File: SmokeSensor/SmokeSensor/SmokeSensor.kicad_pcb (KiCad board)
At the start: 2 copper layers, 88.9 x 59.7 mm, 53 parts, among them J1 USB_C_Receptacle_USB2.0_16P, J2 Conn_01x05_Pin, J3 Conn_01x11, J4 Conn_01x04, Q1 SS8050, Q2 SS8050, SW1 RESET, SW2 BOOT, U1 MT3608, U2 TP4056-42-ESOP8, U3 MCP1700x-330xxMB, U4 CH340C, U5 SHT31-DIS, U6 ESP32-WROOM-32E

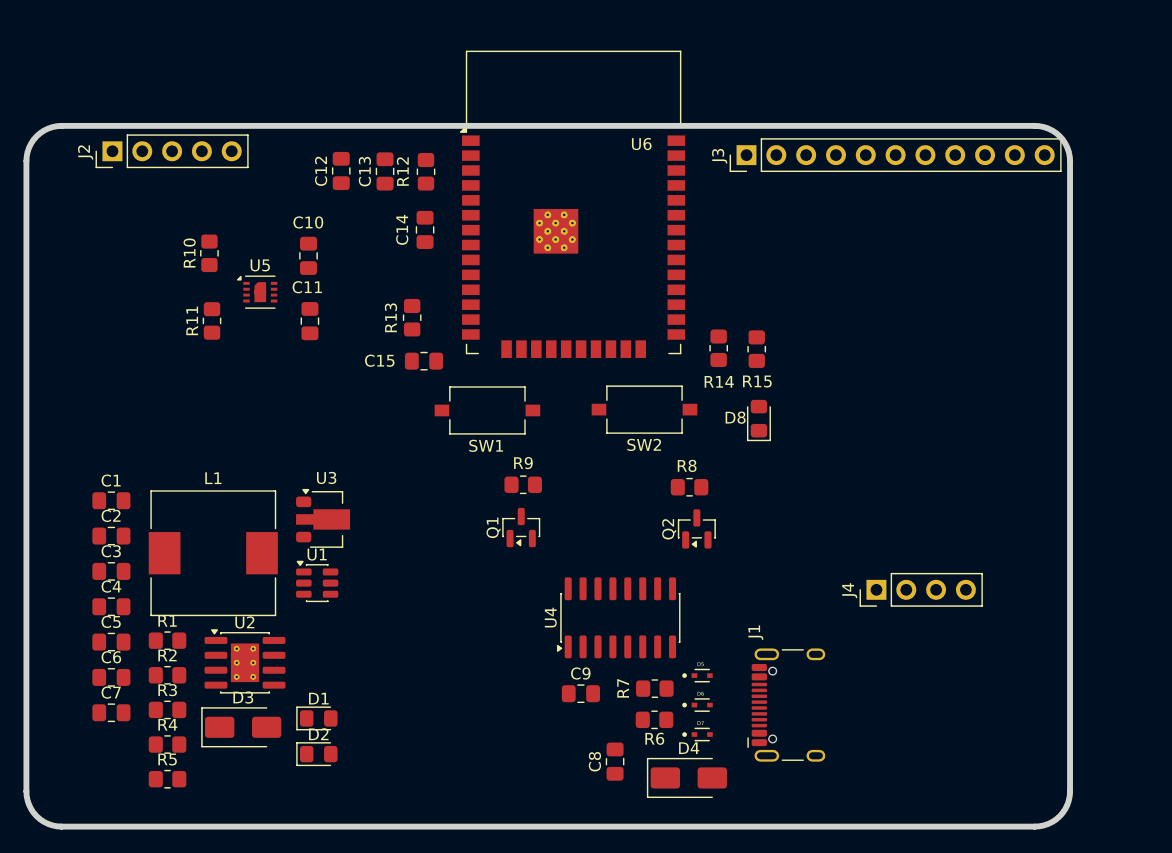
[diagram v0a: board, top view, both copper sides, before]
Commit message: layout 2-layers done!
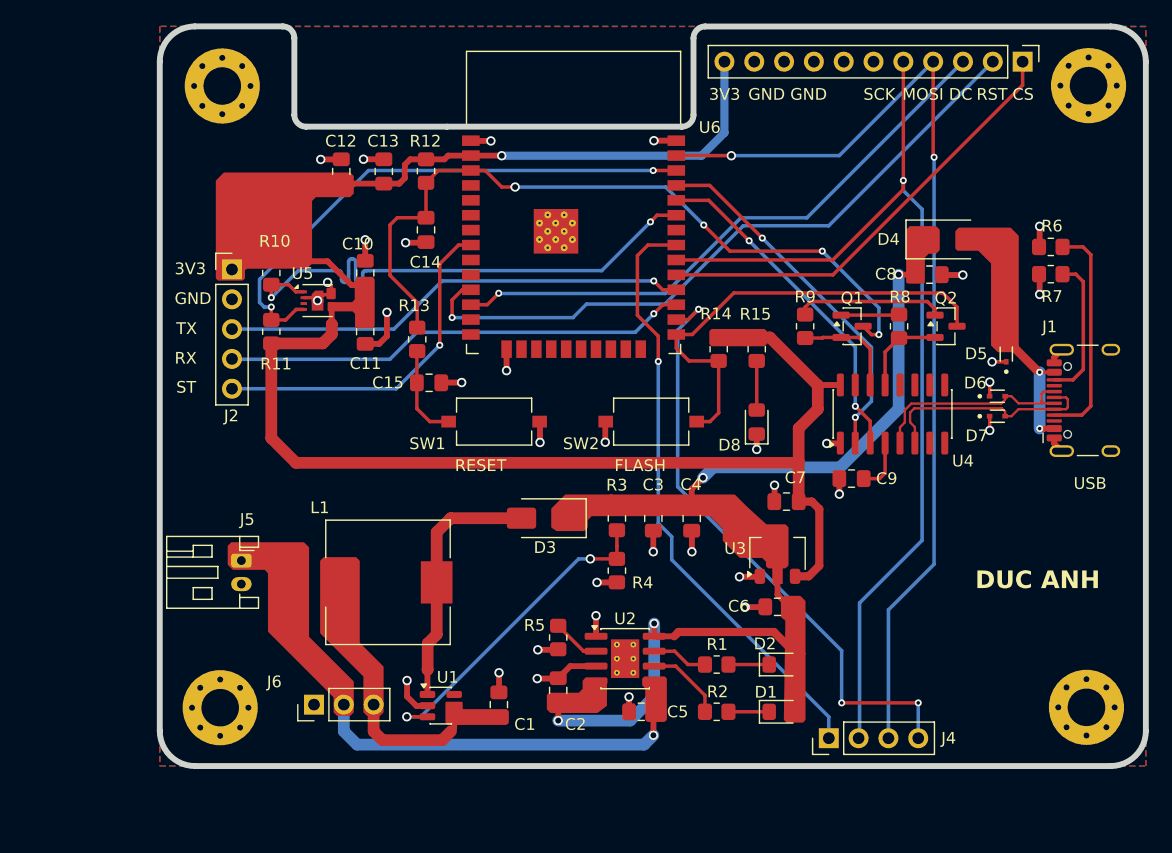
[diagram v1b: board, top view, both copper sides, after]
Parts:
- added J5: Pin lithium, Connector_JST:JST_PH_S2B-PH-K_1x02_P2.00mm_Horizontal, F.Cu at (122.5, 114.5)
- added J6: Switch, Connector_PinHeader_2.54mm:PinHeader_1x03_P2.54mm_Vertical, F.Cu at (128.6, 126.8)
- added REF**: MountingHole_3.2mm_M3_Pad_Via, MountingHole:MountingHole_3.2mm_M3_Pad_Via, F.Cu at (194.6, 74.0)
- added REF**: MountingHole_3.2mm_M3_Pad_Via, MountingHole:MountingHole_3.2mm_M3_Pad_Via, F.Cu at (194.4, 127.0)
- added REF**: MountingHole_3.2mm_M3_Pad_Via, MountingHole:MountingHole_3.2mm_M3_Pad_Via, F.Cu at (120.6, 127.0)
- added REF**: MountingHole_3.2mm_M3_Pad_Via, MountingHole:MountingHole_3.2mm_M3_Pad_Via, F.Cu at (120.8, 74.1)
- L1: value 22uH -> 22uH/2A
- R3: value 1k2 -> 100k
- R4: value 1k2 -> 2k2
- moved C7 60.3 mm to (168.9, 109.5), turned to 180 degrees
- moved C6 57.1 mm to (168.1, 118.4), turned to 180 degrees
- moved R6 52.6 mm to (191.4, 87.8)
- moved D4 50.9 mm to (182.6, 87.1)
- moved C4 50.0 mm to (160.8, 110.9), turned to -90 degrees
- moved C8 49.4 mm to (181.1, 90.1), turned to 0 degrees
- moved R7 48.8 mm to (191.4, 90.1)
- moved R2 46.9 mm to (162.9, 127.4), turned to 180 degrees
- moved R1 46.8 mm to (162.9, 123.4), turned to 180 degrees
- moved C3 46.4 mm to (157.5, 110.9), turned to -90 degrees
- moved C5 45.5 mm to (156.5, 127.4), turned to 180 degrees
- moved R3 41.6 mm to (154.4, 110.9), turned to 90 degrees
- moved R4 41.0 mm to (154.4, 115.4), turned to 90 degrees
- moved C2 40.3 mm to (149.4, 125.6), turned to 90 degrees
- moved D2 40.1 mm to (168.4, 123.4)
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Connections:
- net Net-(U1-EN) renamed /POWER/VBATT/PWR
- net Net-(U2-BAT) renamed /POWER/VBATT
- J3 pad 1: +3.3V -> /ESP32/CS_LCD
- J3 pad 10: /ESP32/RST -> GND
- J3 pad 11: /ESP32/CS_LCD -> +3.3V
- J3 pad 2: GND -> /ESP32/RST
- J3 pad 3: GND -> /ESP32/DC(RS)
- J3 pad 4: unconnected-(J3-Pin_4-Pad4) -> /ESP32/MOSI
- J3 pad 5: unconnected-(J3-Pin_5-Pad5) -> /ESP32/SCK
- J3 pad 7: /ESP32/SCK -> unconnected-(J3-Pin_7-Pad7)
- J3 pad 8: /ESP32/MISO -> unconnected-(J3-Pin_8-Pad8)
- J3 pad 9: /ESP32/DC(RS) -> GND
- J4 pad 3: /ESP32/MISO -> /ESP32/MOSI
- U6 pad 37: /ESP32/MISO -> /ESP32/MOSI
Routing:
- net +3.3V: track 0.00 -> 140.1 mm, vias 0 -> 1
- net /ESP32/MOSI: track 0.00 -> 84.5 mm, vias 0 -> 2
- net /ESP32/SCK: track 0.00 -> 83.1 mm, vias 0 -> 1
- net +5V: track 0.00 -> 69.8 mm, vias 0 -> 4
- net GND: track 0.00 -> 65.9 mm, vias 0 -> 34
- net /ESP32/RESET: track 0.00 -> 63.8 mm, vias 0 -> 4
- net /ESP32/RST: track 0.00 -> 58.6 mm, vias 0 -> 1
- net /ESP32/CS_SD: track 0.00 -> 51.8 mm, vias 0 -> 3
- net /ESP32/MISO: track 0.00 -> 51.5 mm, vias 0 -> 1
- net /ESP32/DC(RS): track 0.00 -> 50.6 mm, vias 0 -> 1
- net /POWER/VBATT: track 0.00 -> 49.1 mm, vias 0 -> 1
- net /ESP32/SCL: track 0.00 -> 46.7 mm, vias 0 -> 2
- net /ESP32/SDA: track 0.00 -> 46.6 mm, vias 0 -> 2
- net /ESP32/Smoke_TX: track 0.00 -> 39.9 mm, vias 0 -> 1
- net /ESP32/Smoke_RX: track 0.00 -> 39.8 mm, vias 0 -> 1
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- added copper zone on B.Cu, net GND
- added copper zone on F.Cu, net GND
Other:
- board size 88.9 x 59.7 mm -> 84 x 63 mm
- board text added: "3V3"
- board text added: "CS"
- board text added: "DC"
- board text added: "DUC ANH"
- board text added: "FLASH"
- board text added: "GND"
- board text added: "MOSI"
- board text added: "RESET"
- board text added: "RST"
- board text added: "RX"
- board text added: "SCK"
- board text added: "ST"
- board text added: "TX"
- board text added: "USB"
